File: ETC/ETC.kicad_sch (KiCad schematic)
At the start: 41 parts, among them CN1 NUCLEO-L432KC, P1 DTM1312PC12PDR008, U2 MCP6004, U3 LM7805_TO220, U4 LM7809_TO220, U6 ISO1050DUB

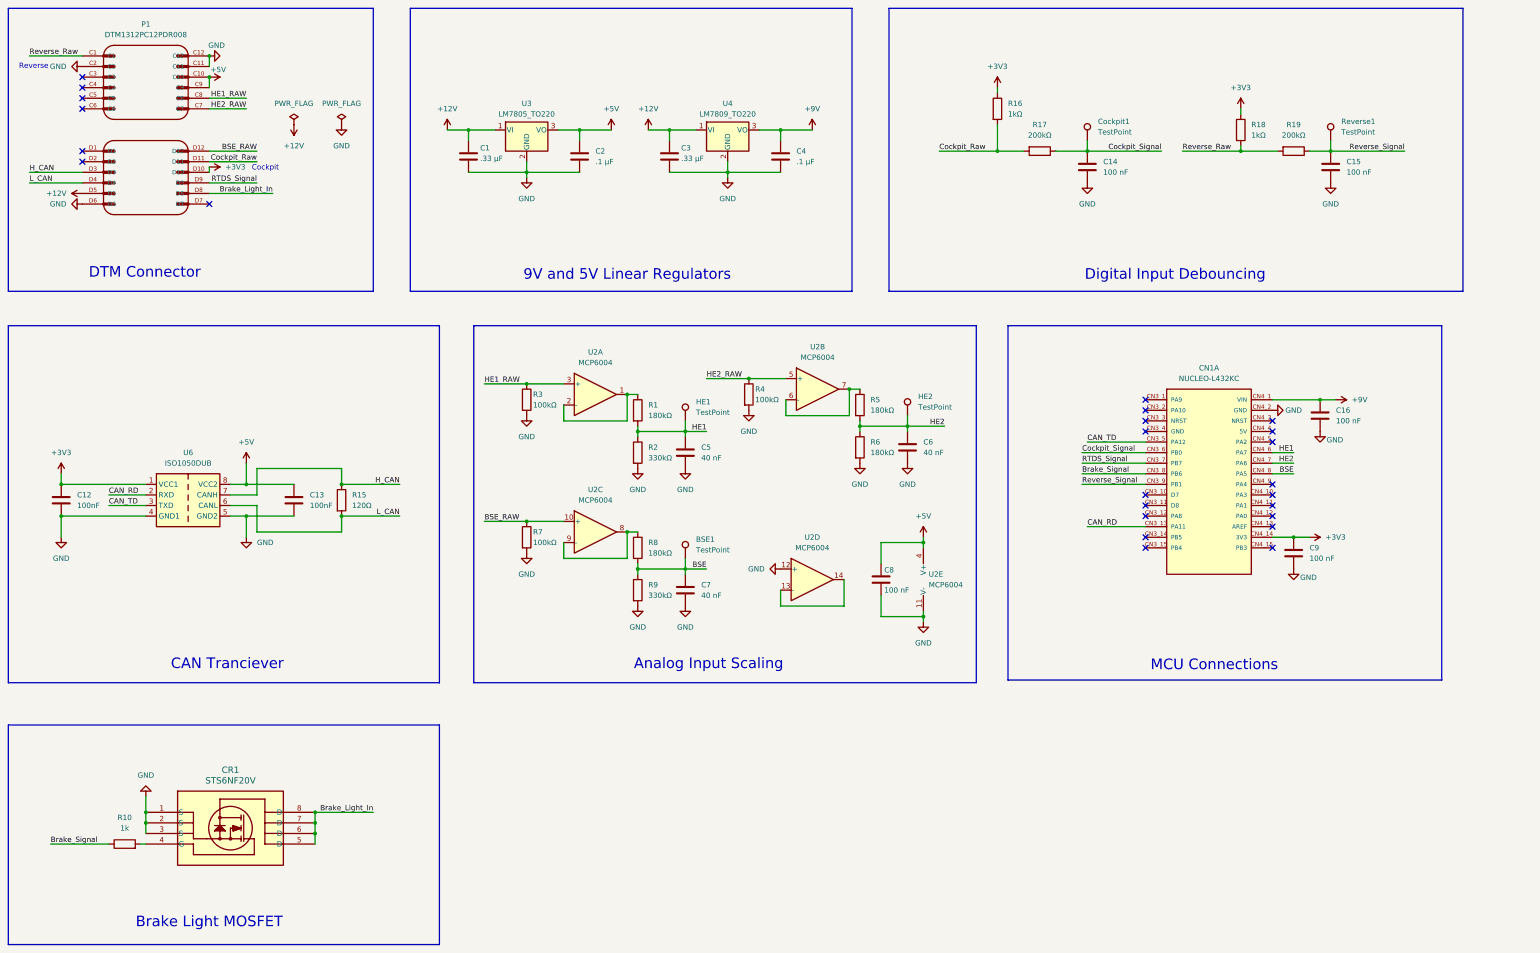
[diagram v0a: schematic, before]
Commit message: Revision 3.1 nanofit headers
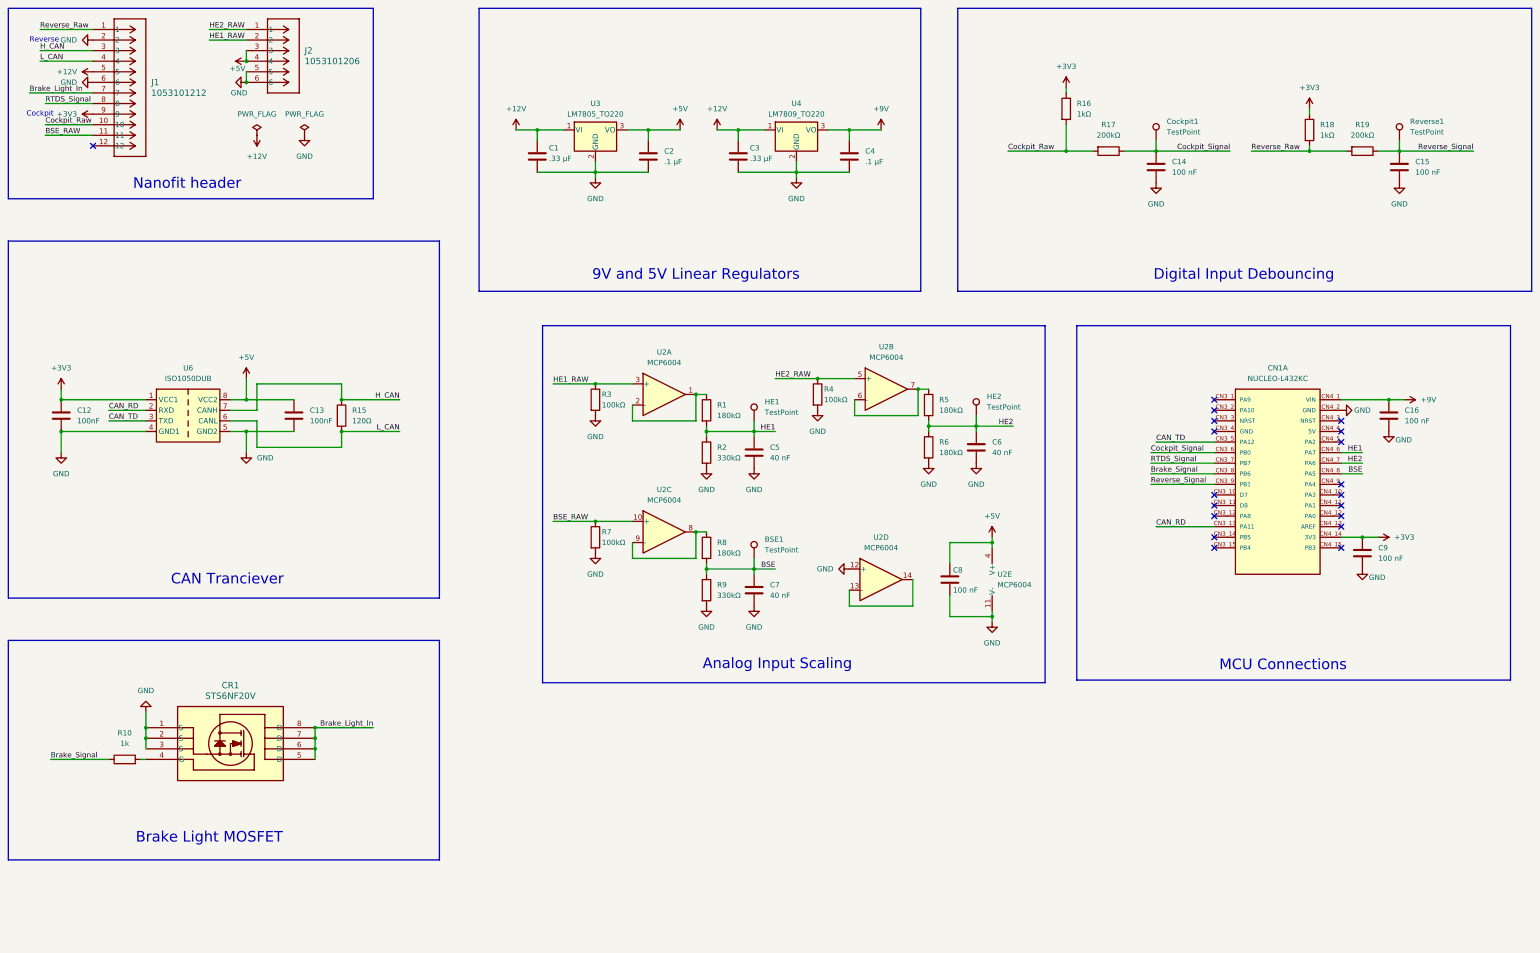
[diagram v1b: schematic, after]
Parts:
- removed P1: DTM1312PC12PDR008, FS_3_Global_Footprint_Library:TE_DTM1312PC12PDR008, symbol FS_3_Global_Symbol_Library:DTM1312PC12PDR008
- added J1: 1053101212, Connector_Molex:Molex_Nano-Fit_105310-xx12_2x06_P2.50mm_Vertical, symbol FS_Symbols:1053101212
- added J2: 1053101206, Connector_Molex:Molex_Nano-Fit_105310-xx06_2x03_P2.50mm_Vertical, symbol FS_Symbols:1053101206
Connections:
- net +12V: now also J1.5
- net +3V3: now also J1.9
- net +5V: now also J2.3, J2.4
- net BSE_RAW: now also J1.11
- net Brake_Light_In: now also J1.7
- net Cockpit_Raw: now also J1.10
- net GND: now also J1.2, J1.6, J2.5, J2.6
- net HE1_RAW: now also J2.2
- net HE2_RAW: now also J2.1
- net H_CAN: now also J1.3
- net L_CAN: now also J1.4
- net RTDS_Signal: now also J1.8
- net Reverse_Raw: now also J1.1
- no-connect marks 25 -> 19
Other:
- note added: "Nanofit header"
- note removed: "DTM Connector"
- moved on the sheet: BSE1, C1, C12, C13, C14, C15, C16, C2, C3, C4, C5, C6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
